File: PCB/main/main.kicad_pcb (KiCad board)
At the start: 2 copper layers, 88.9 x 53.3 mm, 4 parts, among them J1 Conn_01x33_Female, J2 Conn_01x33_Female, J3 Conn_01x33_Female, J4 Conn_01x33_Female

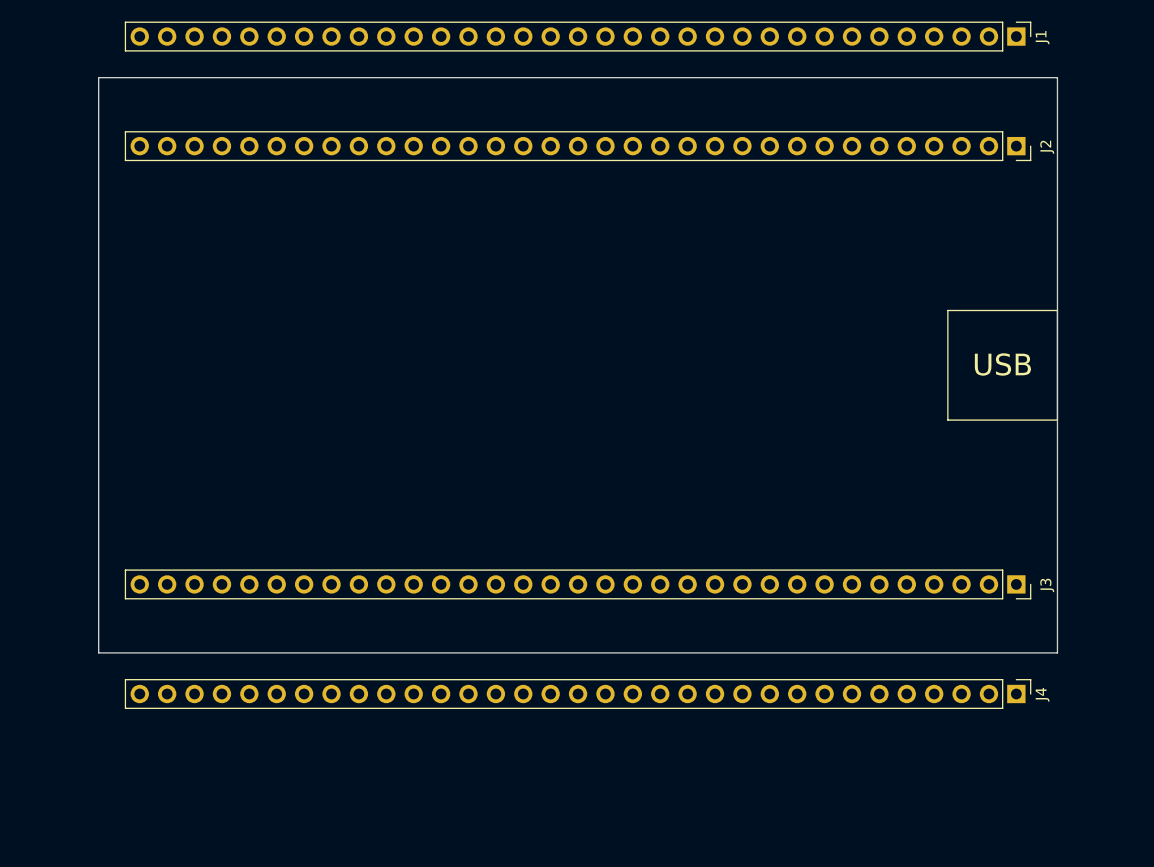
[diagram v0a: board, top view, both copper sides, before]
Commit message: Schematics v0.1.1 & PCB v0.01
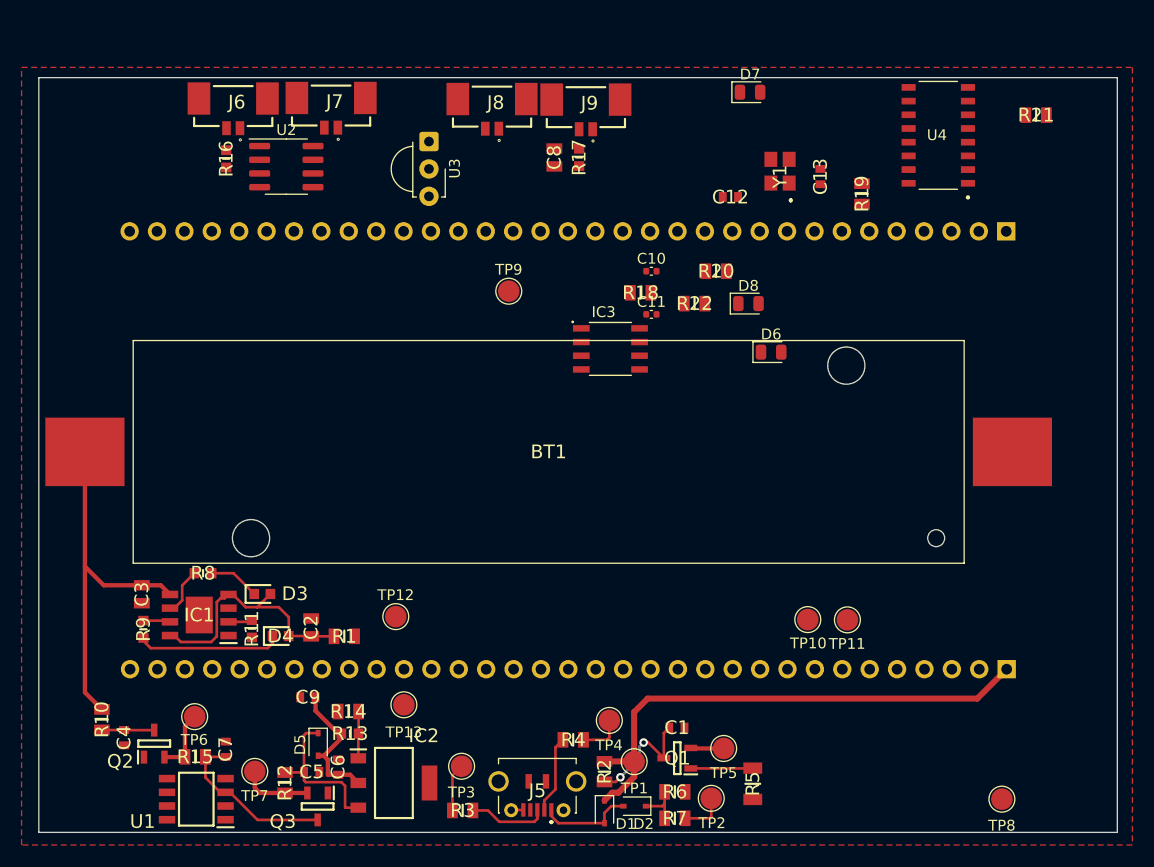
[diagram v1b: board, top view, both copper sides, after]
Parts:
- removed J1, J4: Conn_01x33_Female, Connector_PinHeader_2.54mm:PinHeader_1x33_P2.54mm_Vertical
- added BT1: 18650 Battery, bat_holder:KEYSTONE-1042, F.Cu at (137.0, 104.5)
- added C1: 1u, 1uF_0804:CAPC1608X90N, F.Cu at (148.9, 130.1)
- added C10: 100n, Capacitor_SMD:C_0402_1005Metric, F.Cu at (146.5, 87.8)
- added C11: 100n, Capacitor_SMD:C_0402_1005Metric, F.Cu at (146.5, 91.8)
- added C12: 22p, 22pF_0804:CAPC1608X90N, F.Cu at (153.8, 80.9)
- added C13: 22p, 22pF_0804:CAPC1608X90N, F.Cu at (162.2, 79.0)
- added C2: 10uF, 10uF_0804:CAPC2012X145N, F.Cu at (115.0, 120.8)
- added C3: 10uF, 10uF_0804:CAPC2012X145N, F.Cu at (99.2, 117.8)
- added C4: 1u, 1uF_0804:CAPC1608X90N, F.Cu at (97.6, 131.1)
- added C5: 1u, 1uF_0804:CAPC1608X90N, F.Cu at (115.0, 134.2)
- added C6: 1u, 1uF_0804:CAPC1608X90N, F.Cu at (117.5, 133.8)
- added C7: 1u, 1uF_0804:CAPC1608X90N, F.Cu at (107.0, 132.1)
- added C8: 10uF, 10uF_0804:CAPC2012X145N, F.Cu at (137.5, 77.2)
- added C9: 47n, 47nF_0804:CAPC1608X90N, F.Cu at (114.7, 127.3)
- added D1: 1N5819WS, Diode_SMD:D_SOD-323, F.Cu at (142.2, 137.9)
- added D2: 1N5819WS, Diode_SMD:D_SOD-323, F.Cu at (144.9, 137.4)
- added D3: Green LED, Green_LED:LEDC1608X50N, F.Cu at (110.4, 117.7)
- added D4: Red LED, Red_LED:LEDC1608X70N, F.Cu at (112.1, 121.6)
- added D5: 1N5819WS, Diode_SMD:D_SOD-323, F.Cu at (115.6, 131.7)
- added D6: LED, LED_SMD:LED_0805_2012Metric, F.Cu at (157.6, 95.3)
- added D7: LED, LED_SMD:LED_0805_2012Metric, F.Cu at (155.7, 71.2)
- added D8: LED, LED_SMD:LED_0805_2012Metric, F.Cu at (155.5, 90.8)
- added IC1: TP4056-42-ESOP8, TP4506:SOIC127P600X175-9N, F.Cu at (104.6, 119.7)
- added IC2: AMS1117-3.3, AMS1117-3.3V:SOT229P700X180-4N, F.Cu at (122.6, 135.2)
- added IC3: AT24C256C-SSHL-T, 3088_uC:SOIC127P600X175-8N, F.Cu at (142.7, 95.0)
- added J5: MICROXNJ, MICROXNJ:MICROXNJ, F.Cu at (135.9, 133.0)
- added J6: Conn_01x02_Male, conn_Molex_01_02_vert:53398-0271, F.Cu at (107.7, 74.3)
- added J7: Conn_01x02_Male, conn_Molex_01_02_vert:53398-0271, F.Cu at (116.8, 74.3)
- added J8: Conn_01x02_Male, conn_Molex_01_02_vert:53398-0271, F.Cu at (131.7, 74.4)
- added J9: Conn_01x02_Male, conn_Molex_01_02_vert:53398-0271, F.Cu at (140.4, 74.4)
- added Q1: AO3401A, AO3401A:SOT95P280X125-3N, F.Cu at (148.9, 132.9)
- added Q2: AO3401A, AO3401A:SOT95P280X125-3N, F.Cu at (100.4, 131.6)
- added Q3: AO3401A, AO3401A:SOT95P280X125-3N, F.Cu at (115.5, 137.4)
- added R1: 0R, 0R:RESC2013X65N, F.Cu at (118.0, 121.7)
- added R10: 0R, 0R:RESC2013X65N, F.Cu at (95.5, 129.4)
- added R11: 1k2, 1k:RESC1608X55N, F.Cu at (109.5, 121.0)
- added R12: 0R, 0R:RESC2013X65N, F.Cu at (112.5, 135.2)
- added R13: 3.3k, 3k3:RESC1608X55N, F.Cu at (118.5, 130.7)
- added R14: 4.7k, 4k7:RESC2013X65N, F.Cu at (118.4, 128.6)
- added R15: 0R, 0R:RESC2013X65N, F.Cu at (104.2, 132.8)
- added R16: 1k, 1k:RESC1608X55N, F.Cu at (107.1, 77.4)
- added R17: 1k, 1k:RESC1608X55N, F.Cu at (139.8, 77.2)
- added R18: 4.7k, 4k7:RESC2013X65N, F.Cu at (145.5, 89.8)
- added R19: 4.7k, 4k7:RESC2013X65N, F.Cu at (166.0, 80.6)
- added R2: 0R, 0R:RESC2013X65N, F.Cu at (142.2, 134.2)
- added R20: 1.5k, 4k7:RESC2013X65N, F.Cu at (152.5, 87.8)
- added R21: 1.5k, 4k7:RESC2013X65N, F.Cu at (182.2, 73.3)
- added R22: 1.5k, 4k7:RESC2013X65N, F.Cu at (150.5, 90.8)
- added R3: 0R, 0R:RESC2013X65N, F.Cu at (129.0, 137.8)
- added R4: 0R, 0R:RESC2013X65N, F.Cu at (139.2, 131.2)
- added R5: 100Ω, 100_ohm:RESC3116X65N, F.Cu at (155.9, 135.3)
- added R6: 4.7k, 4k7:RESC2013X65N, F.Cu at (148.7, 136.1)
- added R7: 4.7k, 4k7:RESC2013X65N, F.Cu at (148.7, 138.5)
- added R8: 1kΩ, 1k:RESC1608X55N, F.Cu at (104.9, 115.8)
- added R9: 1kΩ, 1k:RESC1608X55N, F.Cu at (99.4, 121.0)
- added TP1: TestPoint, TestPoint:TestPoint_Pad_D2.0mm, F.Cu at (144.9, 133.3)
- added TP10: TestPoint, TestPoint:TestPoint_Pad_D2.0mm, F.Cu at (161.0, 120.1)
- added TP11: TestPoint, TestPoint:TestPoint_Pad_D2.0mm, F.Cu at (164.7, 120.1)
- added TP12: TestPoint, TestPoint:TestPoint_Pad_D2.0mm, F.Cu at (122.8, 119.8)
- added TP13: TestPoint, TestPoint:TestPoint_Pad_D2.0mm, F.Cu at (123.5, 128.0)
- added TP2: TestPoint, TestPoint:TestPoint_Pad_D2.0mm, F.Cu at (152.1, 136.7)
- added TP3: TestPoint, TestPoint:TestPoint_Pad_D2.0mm, F.Cu at (128.9, 133.7)
- added TP4: TestPoint, TestPoint:TestPoint_Pad_D2.0mm, F.Cu at (142.6, 129.4)
- added TP5: TestPoint, TestPoint:TestPoint_Pad_D2.0mm, F.Cu at (153.2, 132.1)
- added TP6: TestPoint, TestPoint:TestPoint_Pad_D2.0mm, F.Cu at (104.2, 129.1)
- added TP7: TestPoint, TestPoint:TestPoint_Pad_D2.0mm, F.Cu at (109.7, 134.2)
- added TP8: TestPoint, TestPoint:TestPoint_Pad_D2.0mm, F.Cu at (179.0, 136.8)
- added TP9: TestPoint, TestPoint:TestPoint_Pad_D2.0mm, F.Cu at (133.3, 89.7)
- added U1: LM393, LMS393DRG:SOIC127P600X175-8N, F.Cu at (104.3, 136.8)
- added U2: DS18B20Z, Package_SO:SOIC-8_3.9x4.9mm_P1.27mm, F.Cu at (112.7, 78.1)
- added U3: ALS-PDIC15-21B/TR8, OptoDevice:Vishay_MINICAST-3Pin, F.Cu at (125.9, 75.8)
- added U4: CH340G, 3088_uC:SOIC127P600X180-16N, F.Cu at (173.1, 75.2)
- added Y1: YSX321SL, 3088_uC:YSX321SL, F.Cu at (158.4, 78.5)
- J2, J3: moved to B.Cu
- moved J2 7.96 mm to (179.4, 84.1), turned to 90 degrees
- moved J3 7.91 mm to (179.4, 124.7), turned to 90 degrees
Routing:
- net +5V: track 0.00 -> 48.6 mm
- net /Power/BAT +: track 0.00 -> 33.5 mm
- net Net-(C2-Pad1): track 0.00 -> 23.5 mm
- net Net-(C7-Pad1): track 0.00 -> 15.8 mm
- net Net-(C5-Pad1): track 0.00 -> 14.6 mm
- net Net-(D4-Pad1): track 0.00 -> 13.4 mm
- net +3V0: track 0.00 -> 12.8 mm
- net Net-(C1-Pad1): track 0.00 -> 11.3 mm, vias 0 -> 2
- net Net-(D1-Pad2): track 0.00 -> 8.73 mm
- net Net-(J5-Pad3): track 0.00 -> 7.35 mm
- net Net-(J5-Pad2): track 0.00 -> 7.21 mm
- net /Power/UVLO_OUT: track 0.00 -> 6.60 mm
- net /Power/BATOUT: track 0.00 -> 6.01 mm
- net Net-(Q1-Pad1): track 0.00 -> 5.76 mm
- net Net-(C4-Pad1): track 0.00 -> 4.86 mm
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- added copper zone on F.Cu, net GND
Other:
- board size 88.9 x 53.3 mm -> 100 x 70 mm
- board text removed: "USB"
